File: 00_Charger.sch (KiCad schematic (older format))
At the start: 42 parts, among them J401 Jack-DC, Q401 NTK3043N, Q402 FDD4685-F085, U401 MAX1873TEEE, U402 PC827

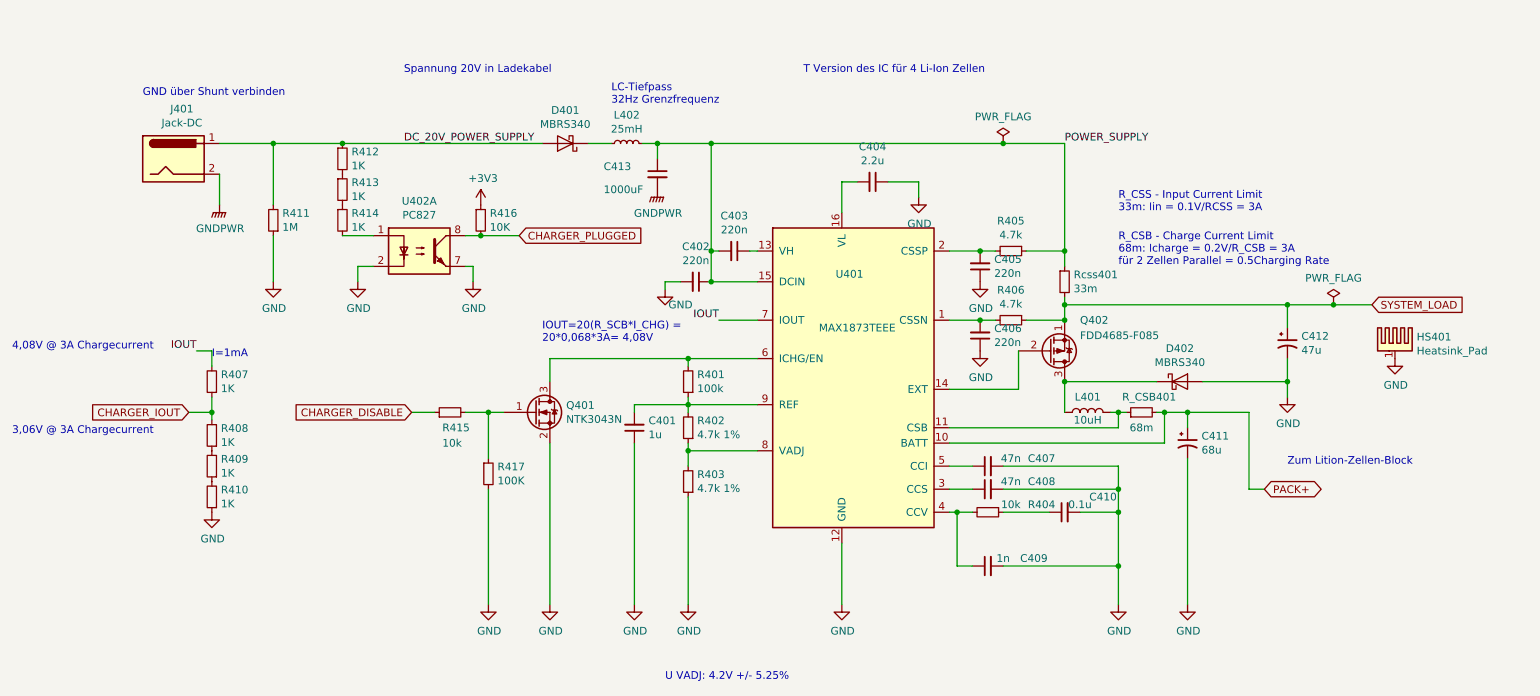
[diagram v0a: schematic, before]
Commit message: fast alle footprints herausgesucht. Spulen typen rausgesucht: Bourns spulen
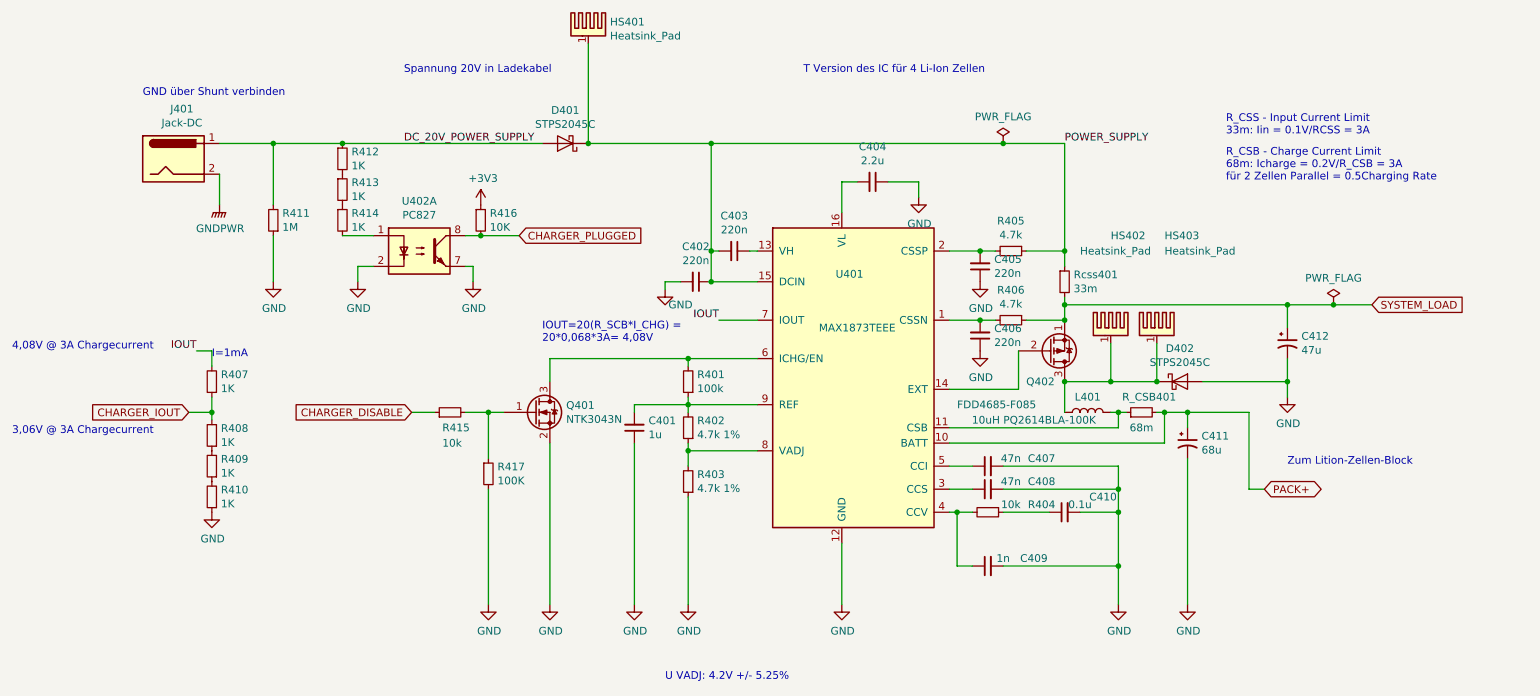
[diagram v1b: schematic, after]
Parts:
- removed C413: 1000uF, Capacitor_SMD:CP_Elec_16x17.5, symbol Device:C_Small
- removed L402: 25mH, symbol Device:L_Small
- added HS402, HS403: Heatsink_Pad, Heatsink:Heatsink_AAVID_573300D00010G_TO-263, symbol Mechanical:Heatsink_Pad
- D401, D402: value MBRS340 -> STPS2045C; footprint (none) -> Package_TO_SOT_SMD:TO-263-2
- HS401: footprint (none) -> Heatsink:Heatsink_AAVID_573300D00010G_TO-263
- L401: value 10uH -> 10uH PQ2614BLA-100K; footprint (none) -> Inductor_SMD:PQ2617BHA-330K
- Q401: footprint (none) -> Package_TO_SOT_SMD:SOT-723
- Q402: footprint (none) -> Package_TO_SOT_SMD:TO-263-2
- R401, R402, R403, R404, R405, R406, R407, R408, R409, R410, R411, R412, R413, R414, R415, R416, R417: footprint (none) -> Resistor_SMD:R_0603_1608Metric_Pad1.05x0.95mm_HandSolder
- R_CSB401, Rcss401: footprint (none) -> Resistor_SMD:R_1206_3216Metric_Pad1.42x1.75mm_HandSolder
- U402: footprint Package_DIP:DIP-8_W7.62mm -> Package_DIP:DIP-8_W7.62mm_SMDSocket_SmallPads
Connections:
- net GND: no longer HS401.1
- net POWER_SUPPLY: now also D401.1 (K), HS401.1
- net at D402.1 (K), L401.1, Q402.3 (D): now also HS402.1, HS403.1
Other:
- note removed: "LC-Tiefpass\n32Hz Grenzfrequenz"
